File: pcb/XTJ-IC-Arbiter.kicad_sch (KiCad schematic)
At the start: 58 parts, among them IC1 TLV3704IN, J3 DTM13-12PA-R008, U1 LM2675N-5.0/NOPB, U2 CDP68HC68S1, U3 EEC-325X4A, U4 MCP2562-H-P, U5 SP723APP, U6 MCP1700-3302E/TO, U7 DS18B20

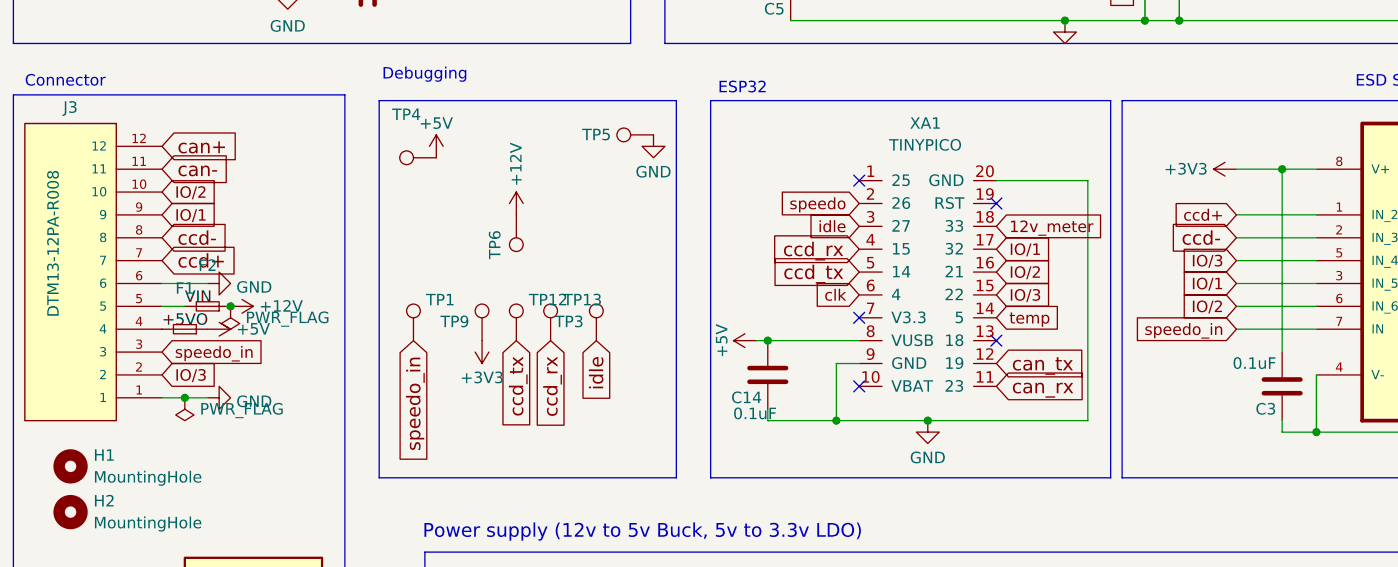
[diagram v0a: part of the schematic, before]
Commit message: improve clearance
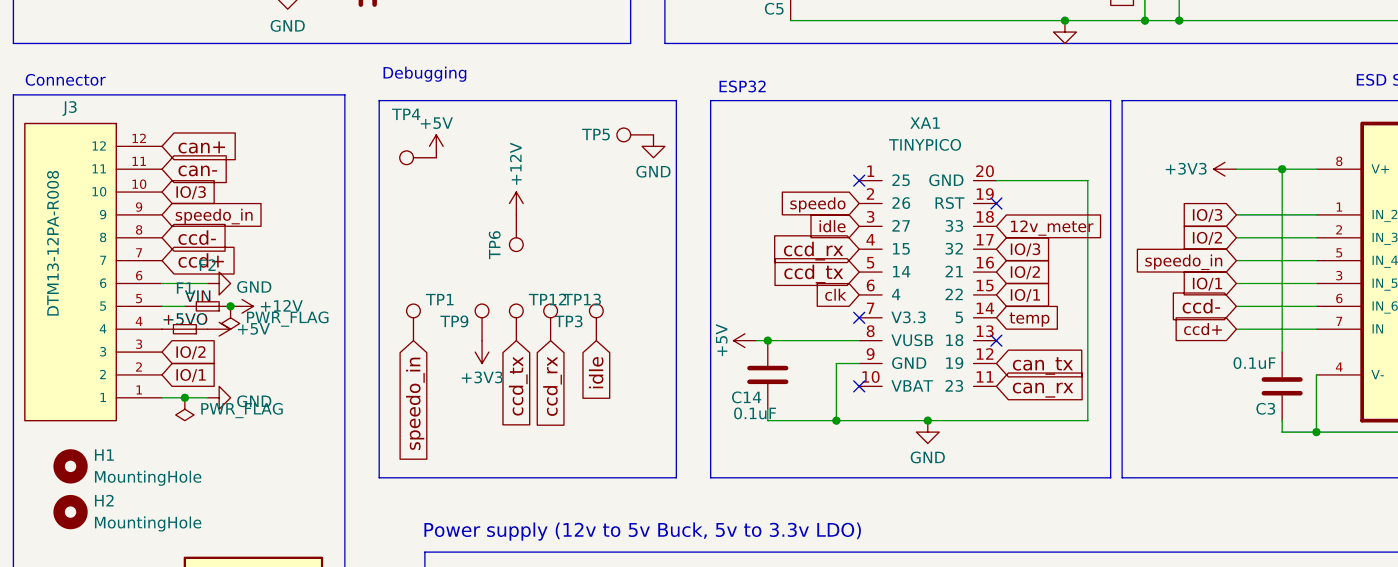
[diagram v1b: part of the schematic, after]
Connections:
- net IO/1: now also J3.2, XA1.15 (22); no longer J3.9, XA1.17 (32)
- net IO/2: now also J3.3, U5.2 (IN_3); no longer J3.10, U5.6 (IN_6)
- net IO/3: now also J3.10, U5.1 (IN_2), XA1.17 (32); no longer J3.2, U5.5 (IN_4), XA1.15 (22)
- net ccd+: now also U5.7 (IN); no longer U5.1 (IN_2)
- net ccd-: now also U5.6 (IN_6); no longer U5.2 (IN_3)
- net speedo_in: now also J3.9, U5.5 (IN_4); no longer J3.3, U5.7 (IN)
